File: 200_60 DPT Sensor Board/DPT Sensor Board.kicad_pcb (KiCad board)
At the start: 2 copper layers, 15 x 15 mm, 2 parts, among them J1 5034800640

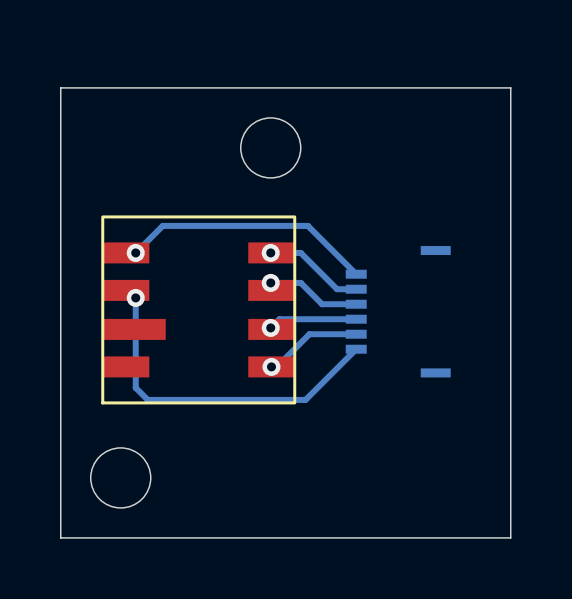
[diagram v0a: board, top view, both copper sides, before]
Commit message: completed dpt board & discharge:
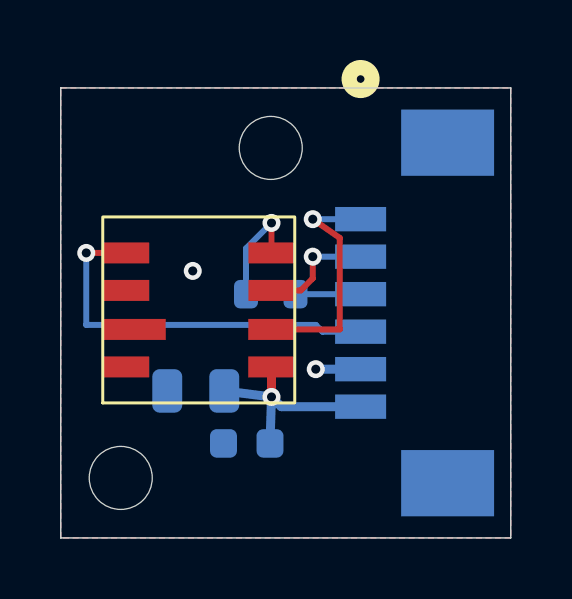
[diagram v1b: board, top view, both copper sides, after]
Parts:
- added C1: 100nF, Capacitor_SMD:C_0603_1608Metric, B.Cu at (155.2, 101.3)
- added C2: 10uF, Capacitor_SMD:C_0805_2012Metric, B.Cu at (153.5, 99.6)
- added H1: MountingHole, MountingHole:MountingHole_2.1mm, F.Cu at (151.0, 102.5)
- added H2: MountingHole, MountingHole:MountingHole_2.1mm, F.Cu at (156.0, 91.5)
- added R1: 22, Resistor_SMD:R_0603_1608Metric, B.Cu at (156.0, 96.4)
- J1: value 5034800640 -> 53261-0671; footprint 0_PAY_Footprint_Library:CON_5034800640_MOL -> 0_PAY_Footprint_Library:CONN_532610001-SD_06_MOL
- U1: value ~ -> MS5540C
- moved J1 1.55 mm to (161.9, 97.0), turned to 90 degrees
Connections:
- J1 pad 1: Net-(U1-SCLK) -> Net-(U1-MCLK)
- J1 pad 2: Net-(U1-DOUT) -> Net-(U1-DIN)
- J1 pad 3: Net-(U1-DIN) -> Net-(J1-Pad3)
- J1 pad 4: Net-(U1-MCLK) -> /SCLK
- J1 pad 5: Net-(U1-VDD) -> GND
- J1 pad 6: Net-(U1-GND) -> +3.3V
- U1 pad 1: Net-(U1-SCLK) -> /SCLK
- U1 pad 2: Net-(U1-GND) -> GND
- U1 pad 5: Net-(U1-VDD) -> +3.3V
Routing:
- net /SCLK: track 0.00 -> 13.0 mm, vias 0 -> 1
- net Net-(U1-GND): track 11.6 -> 0.00 mm, vias 1 -> 0
- net Net-(U1-SCLK): track 8.71 -> 0.00 mm, vias 1 -> 0
- net +3.3V: track 0.00 -> 7.24 mm, vias 0 -> 1
- net Net-(U1-MCLK): track 3.03 -> 8.02 mm
- net Net-(U1-VDD): track 3.28 -> 0.00 mm, vias 1 -> 0
- net Net-(J1-Pad3): track 0.00 -> 2.17 mm
- net GND: track 0.00 -> 1.50 mm, vias 0 -> 2
- added copper zone on B.Cu, net GND
- added copper zone on F.Cu, net GND
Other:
- outline, holes or cut-outs redrawn
- board text added: "DPT john"
- board text removed: "DPT Board"

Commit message: DPT cleanup
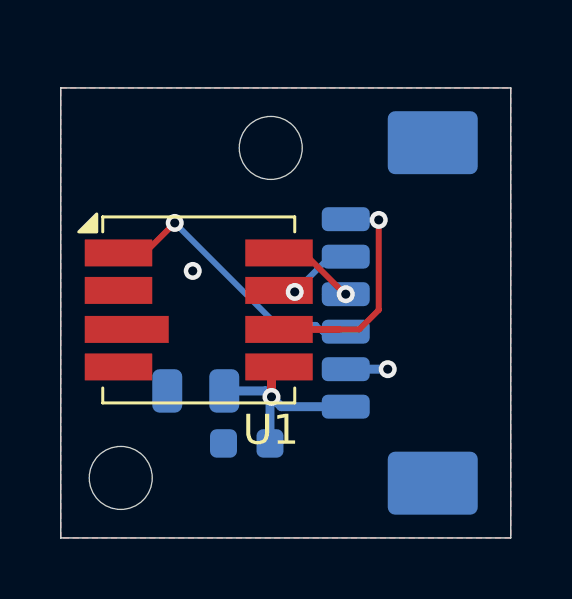
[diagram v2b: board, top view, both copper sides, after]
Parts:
- removed R1: 22, Resistor_SMD:R_0603_1608Metric
- J1: value 53261-0671 -> Conn_01x06_MountingPin; footprint 0_PAY_Footprint_Library:CONN_532610001-SD_06_MOL -> Connector_Molex:Molex_PicoBlade_53261-0671_1x06-1MP_P1.25mm_Horizontal
- moved U1 4.46 mm to (153.6, 96.9)
- moved J1 1.00 mm to (160.9, 97.0), turned to -90 degrees
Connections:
- J1 pad 3: Net-(J1-Pad3) -> Net-(J1-Pin_3)
- U1 pad 8: Net-(U1-DOUT) -> Net-(J1-Pin_3)
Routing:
- net Net-(J1-Pin_3): track 0.00 -> 3.74 mm, vias 0 -> 1
- net Net-(U1-DOUT): track 3.73 -> 0.00 mm, vias 1 -> 0
- net /SCLK: track 13.0 -> 9.74 mm
- net Net-(J1-Pad3): track 2.17 -> 0.00 mm
- net Net-(J1-Pin_1): track 8.02 -> 9.98 mm
- net Net-(J1-Pin_2): track 3.86 -> 2.73 mm
- net GND: track 1.50 -> 0.91 mm
